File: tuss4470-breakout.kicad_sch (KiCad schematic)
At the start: 23 parts, among them J1 Screw_Terminal_01x02, J2 Conn_01x08_Pin, J3 Conn_01x08_Pin, J4 Screw_Terminal_01x02, U1 LP5907MFX-3.3, U2 TUSS4470

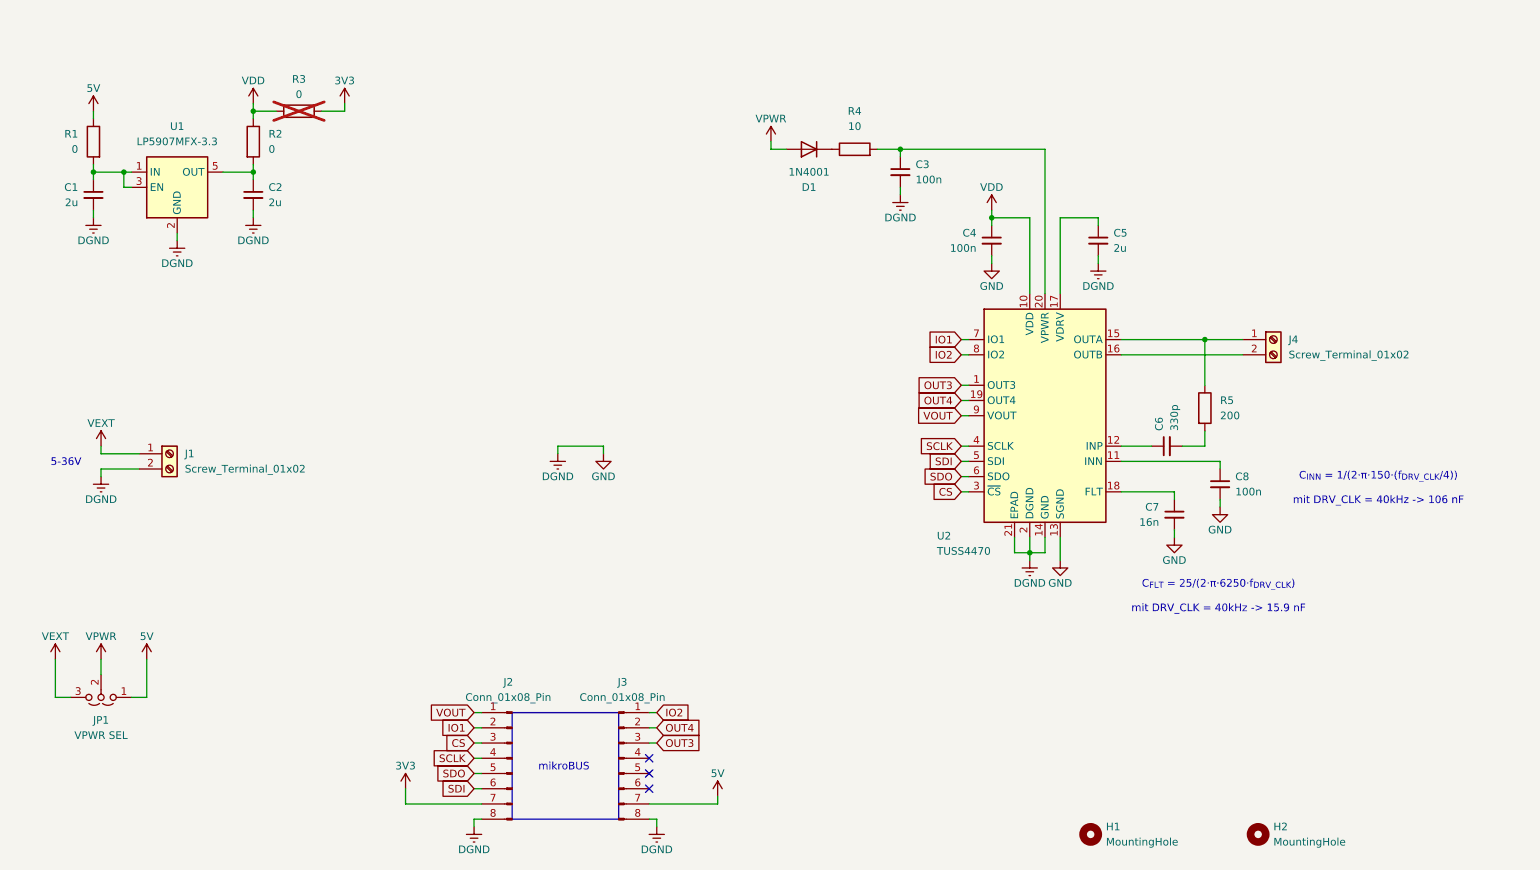
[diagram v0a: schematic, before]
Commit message: generate gerbers
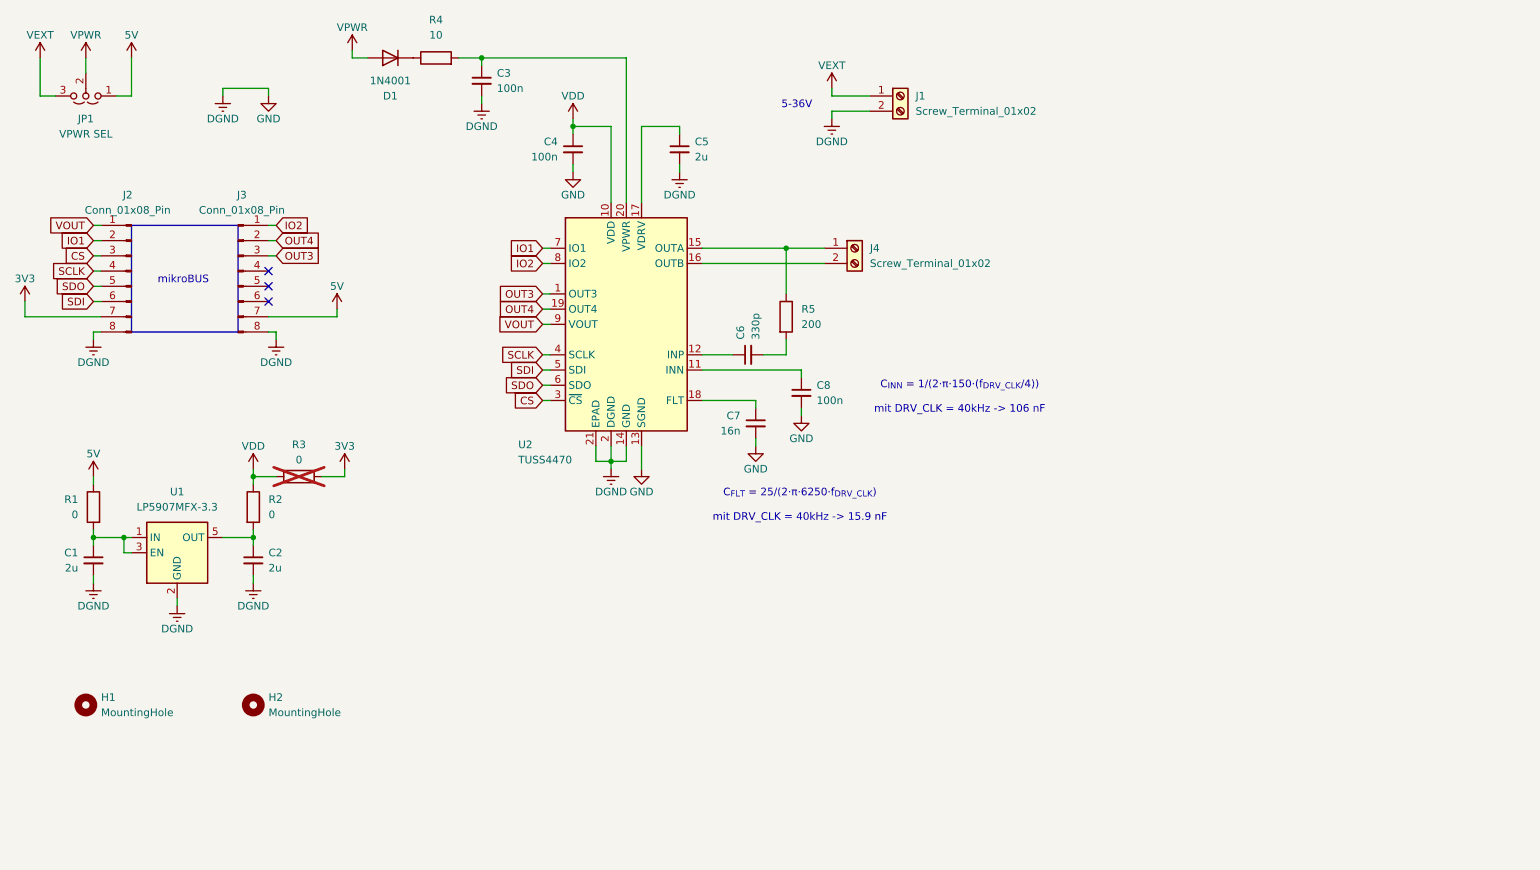
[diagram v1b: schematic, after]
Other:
- company: (none) -> Maximilian Weber
- title: (none) -> TUSS4470 Breakout Board
- moved on the sheet: C1, C2, C3, C4, C5, C6, C7, C8, D1, H1, H2, J1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
